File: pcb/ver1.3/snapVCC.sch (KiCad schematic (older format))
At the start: 16 parts, among them J1 Jumper Shunt, P1 CONN_01X03, P2 CONN_01X02, Q1 IRLML9301TRPbF, U1 TPS560200

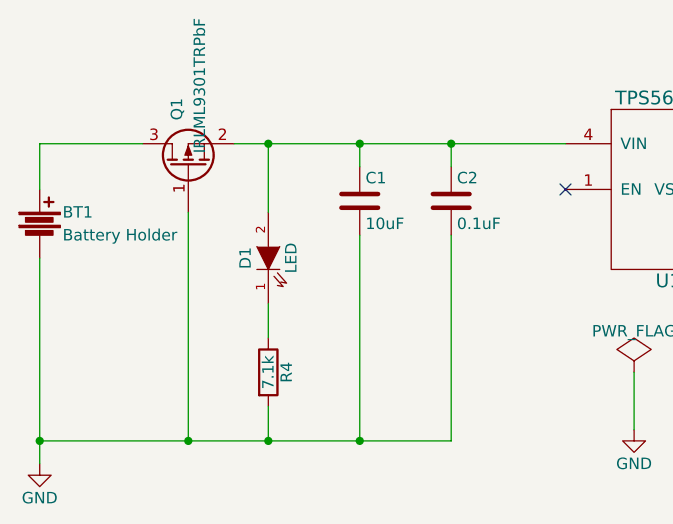
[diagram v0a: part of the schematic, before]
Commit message: ver2.1 updated
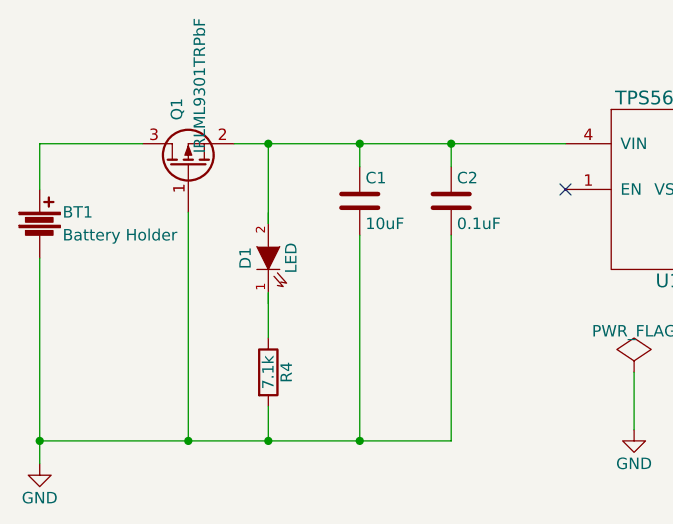
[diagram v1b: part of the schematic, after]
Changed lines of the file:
@@
 EESchema Schematic File Version 2
+LIBS:snapVCC-rescue
 LIBS:power
 LIBS:device
@@
 NoConn ~ 6850 4750
 Wire Wire Line
-	3500 4000 3500 3700
+	3500 3700 3500 4050
 Connection ~ 3500 3700
 Wire Wire Line
@@
 Connection ~ 3500 5000
 Wire Wire Line
-	3500 4400 3500 4550
+	3500 4350 3500 4550
 $EndSCHEMATC
